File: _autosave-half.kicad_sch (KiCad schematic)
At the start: 88 parts, among them J3 JST_PH, Q1 Q_PMOS_GSD, SW1 SW_Push, SW13 SW_Push, SW14 SW_Push, SW15 SW_Push, SW16 SW_Push, SW17 SW_Push, SW18 SW_Push, SW25 SW_Push, SW26 SW_Push, SW27 SW_Push, SW28 SW_Push, SW29 SW_Push, SW3 SW_Push, SW30 SW_Push, SW37 SW_Push, SW38 SW_Push, SW39 SW_Push, SW40 SW_Push, SW41 SW_Push, SW42 SW_Push, SW49 SW_Push, SW5 SW_Push, SW50 SW_Push, SW51 SW_Push, SW52 SW_Push, SW53 SW_Push, SW54 RotaryEncoder_Switch, SW61 SW_SPDT, SW7 SW_Push, SW8 SW_Push, SW9 SW_Push, U3 SuperMini nRF52840

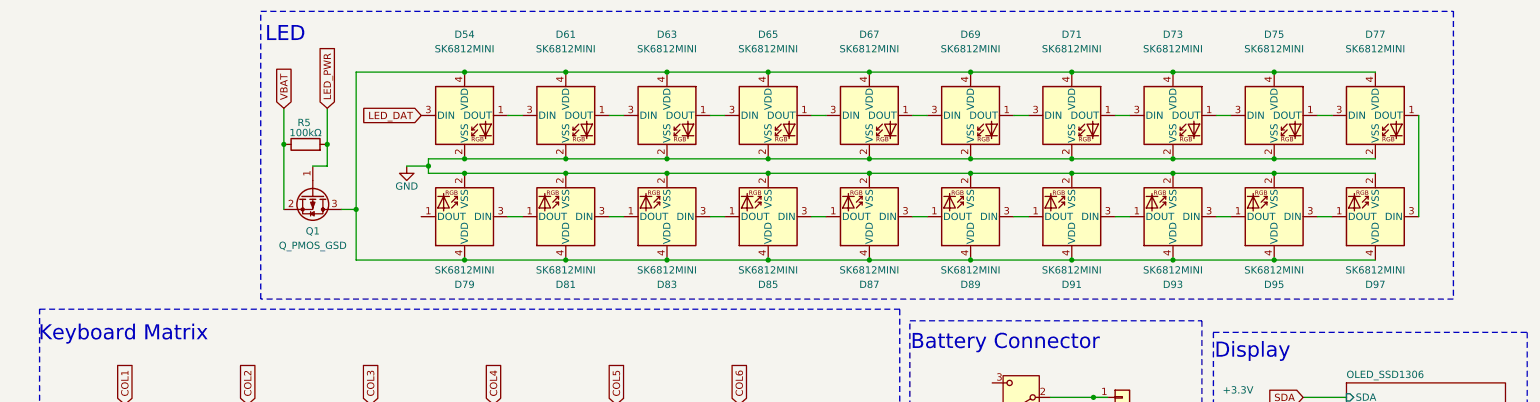
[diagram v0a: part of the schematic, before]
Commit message: update
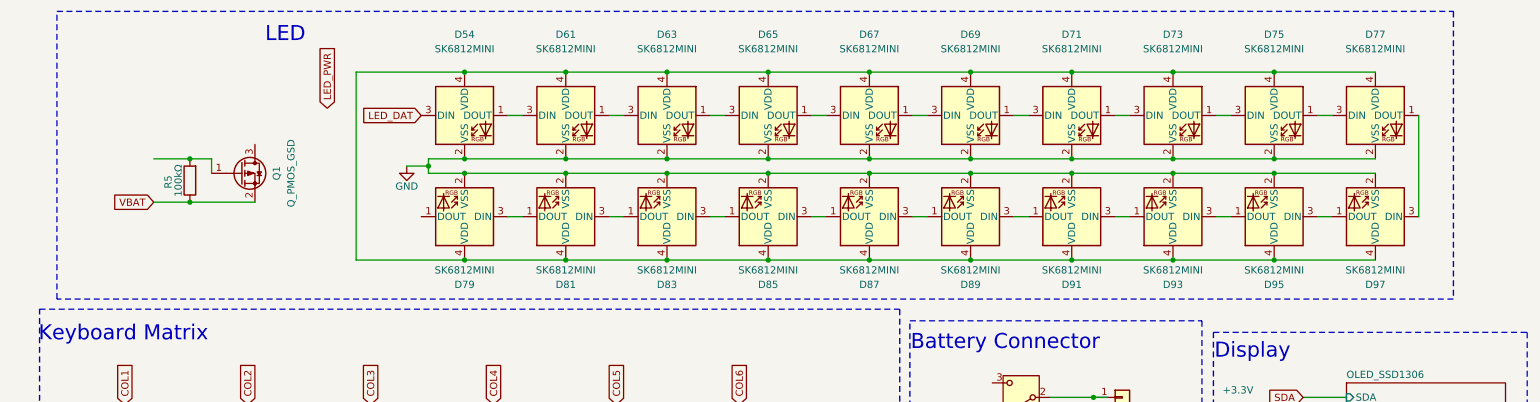
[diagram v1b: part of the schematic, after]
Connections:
- net LED_PWR: no longer Q1.1 (G), R5.2
- net at D54.4 (VDD), D61.4 (VDD), D63.4 (VDD)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: no longer Q1.3 (D)
- new net: Q1.1 (G), R5.2
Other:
- moved on the sheet: Q1, R5
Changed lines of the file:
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@@
 	)
 	(rectangle
-		(start 55.626 16.002)
+		(start 19.812 16.002)
 		(end 265.176 66.548)
 		(stroke
@@
 	)
 	(junction
-		(at 67.31 39.37)
+		(at 43.18 41.91)
 		(diameter 0)
 		(color 0 0 0 0)
@@
 	)
 	(junction
-		(at 59.69 39.37)
+		(at 43.18 49.53)
 		(diameter 0)
 		(color 0 0 0 0)
@@
 	)
 	(junction
-		(at 72.39 50.8)
-		(diameter 0)
-		(color 0 0 0 0)
-	)
-	(junction
 		(at 128.27 140.97)
 		(diameter 0)
@@
 	(wire
 		(pts
-			(xy 69.85 50.8) (xy 72.39 50.8)
-		)
-		(stroke
-			(width 0)
-			(type default)
-		)
-	)
-	(wire
-		(pts
 			(xy 91.44 26.67) (xy 72.39 26.67)
 		)
@@
 	(wire
 		(pts
-			(xy 59.69 33.02) (xy 59.69 39.37)
-		)
-		(stroke
-			(width 0)
-			(type default)
-		)
-	)
-	(wire
-		(pts
-			(xy 72.39 26.67) (xy 72.39 50.8)
+			(xy 36.83 49.53) (xy 43.18 49.53)
 		)
 		(stroke
@@
 	(wire
 		(pts
-			(xy 59.69 39.37) (xy 59.69 50.8)
+			(xy 43.18 49.53) (xy 54.61 49.53)
 		)
 		(stroke
@@
 	(wire
 		(pts
-			(xy 67.31 33.02) (xy 67.31 39.37)
+			(xy 36.83 41.91) (xy 43.18 41.91)
 		)
 		(stroke
@@
 	(wire
 		(pts
-			(xy 67.31 43.18) (xy 67.31 39.37)
+			(xy 46.99 41.91) (xy 43.18 41.91)
 		)
 		(stroke
@@
 	(wire
 		(pts
-			(xy 64.77 43.18) (xy 67.31 43.18)
+			(xy 46.99 44.45) (xy 46.99 41.91)
 		)
 		(stroke
@@
 	(wire
 		(pts
-			(xy 72.39 50.8) (xy 72.39 59.69)
+			(xy 72.39 26.67) (xy 72.39 59.69)
 		)
 		(stroke
@@
 	(global_label "VBAT"
 		(shape input)
-		(at 59.69 33.02 90)
+		(at 36.83 49.53 180)
 		(fields_autoplaced yes)
 		(effects
@@
 				(size 1.27 1.27)
 			)
-			(justify left)
+			(justify right)
 		)
 		(property "Intersheetrefs" "${INTERSHEET_REFS}"
-			(at 59.69 25.62 90)
+			(at 29.43 49.53 0)
 			(effects
 				(font
 					(size 1.27 1.27)
 				)
-				(justify left)
+				(justify right)
 				(hide yes)
 			)
@@
 	(symbol
 		(lib_id "Transistor_FET:Q_PMOS_GSD")
-		(at 64.77 48.26 270)
+		(at 52.07 44.45 0)
 		(unit 1)
 		(exclude_from_sim no)
@@
 		(fields_autoplaced yes)
 		(property "Reference" "Q1"
-			(at 64.77 54.61 90)
+			(at 58.42 44.45 90)
 			(effects
 				(font
@@
 		)
 		(property "Value" "Q_PMOS_GSD"
-			(at 64.77 57.15 90)
+			(at 60.96 44.45 90)
 			(effects
 				(font
@@
 		)
 		(property "Footprint" ""
-			(at 67.31 53.34 0)
+			(at 57.15 41.91 0)
 			(effects
 				(font
@@
 		)
 		(property "Datasheet" "~"
-			(at 64.77 48.26 0)
+			(at 52.07 44.45 0)
 			(effects
 				(font
@@
 		)
 		(property "Description" "P-MOSFET transistor, gate/source/drain"
-			(at 64.77 48.26 0)
+			(at 52.07 44.45 0)
 			(effects
 				(font
@@
 	(symbol
 		(lib_id "Device:R")
-		(at 63.5 39.37 90)
+		(at 43.18 45.72 180)
 		(unit 1)
 		(exclude_from_sim no)
@@
 		(dnp no)
 		(property "Reference" "R5"
-			(at 63.246 35.56 90)
+			(at 39.37 45.974 90)
 			(effects
 				(font
@@
 		)
 		(property "Value" "100kΩ"
-			(at 63.5 37.338 90)
+			(at 41.148 45.72 90)
 			(effects
 				(font
@@
 		)
 		(property "Footprint" "Resistor_SMD:R_0805_2012Metric"
-			(at 63.5 41.148 90)
+			(at 44.958 45.72 90)
 			(effects
 				(font
@@
 		)
 		(property "Datasheet" "~"
-			(at 63.5 39.37 0)
+			(at 43.18 45.72 0)
 			(effects
 				(font
@@
 		)
 		(property "Description" "Resistor"
-			(at 63.5 39.37 0)
+			(at 43.18 45.72 0)
 			(effects
 				(font
